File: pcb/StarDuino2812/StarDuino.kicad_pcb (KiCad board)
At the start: 2 copper layers, 126.3 x 120.3 mm, 68 parts, among them J1 Screw_Terminal_01x02, Q1 IRLML6401, U1 ATmega328P-AU, Y1 Crystal

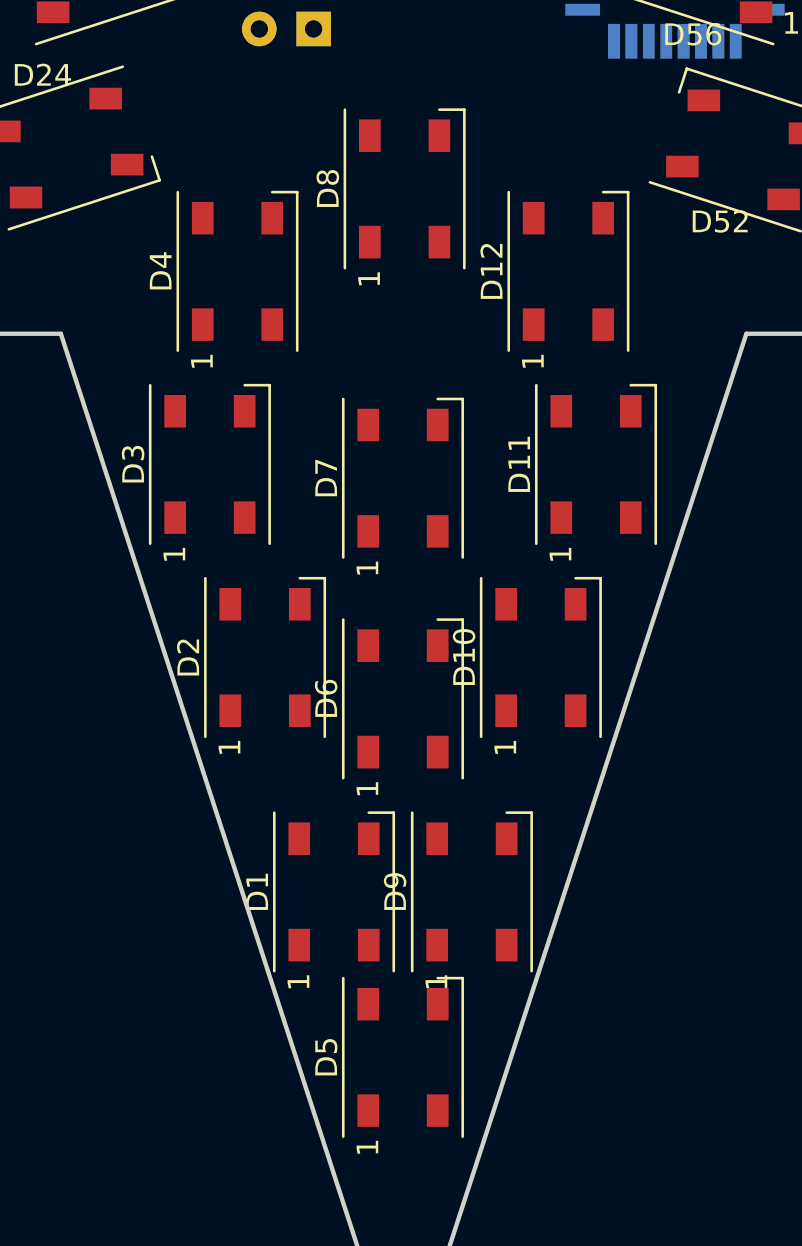
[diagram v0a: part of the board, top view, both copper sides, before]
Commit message: 2812 star in work
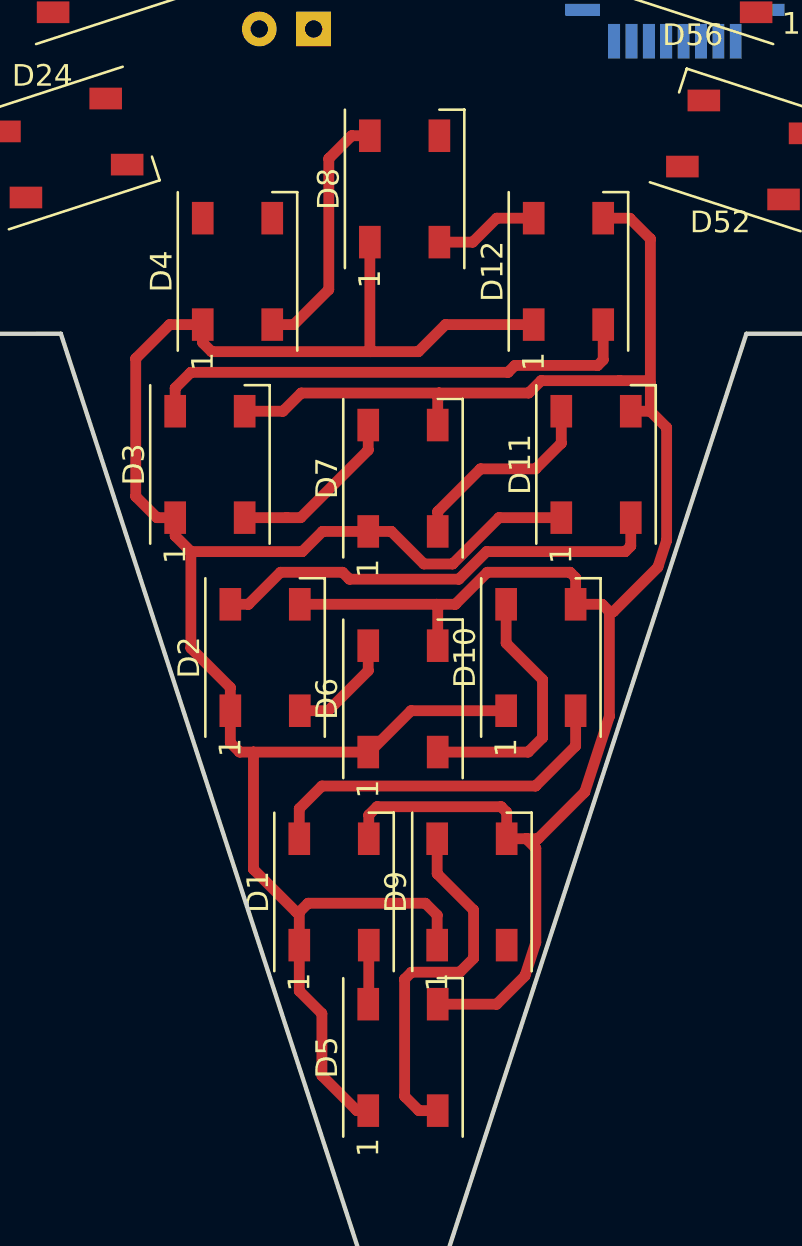
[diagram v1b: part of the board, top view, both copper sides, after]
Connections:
- D10 pad 2: Net-(D10-Pad2) -> Net-(D1-Pad4)
- D11 pad 4: Net-(D10-Pad2) -> Net-(D11-Pad4)
- D12 pad 4: Net-(D11-Pad2) -> Net-(D12-Pad4)
- D14 pad 4: Net-(D13-Pad2) -> Net-(D14-Pad4)
- D15 pad 4: Net-(D14-Pad2) -> Net-(D15-Pad4)
- D16 pad 4: Net-(D15-Pad2) -> Net-(D16-Pad4)
- D18 pad 4: Net-(D17-Pad2) -> Net-(D18-Pad4)
- D19 pad 4: Net-(D18-Pad2) -> Net-(D19-Pad4)
- D2 pad 4: Net-(D1-Pad2) -> Net-(D11-Pad2)
- D20 pad 4: Net-(D19-Pad2) -> Net-(D20-Pad4)
- D22 pad 4: Net-(D21-Pad2) -> Net-(D22-Pad4)
- D23 pad 4: Net-(D22-Pad2) -> Net-(D23-Pad4)
- D24 pad 4: Net-(D23-Pad2) -> Net-(D24-Pad4)
- D26 pad 4: Net-(D25-Pad2) -> Net-(D26-Pad4)
- D27 pad 4: Net-(D26-Pad2) -> Net-(D27-Pad4)
- D28 pad 4: Net-(D27-Pad2) -> Net-(D28-Pad4)
- D3 pad 4: Net-(D2-Pad2) -> Net-(D12-Pad2)
- D30 pad 4: Net-(D29-Pad2) -> Net-(D30-Pad4)
- D31 pad 4: Net-(D30-Pad2) -> Net-(D31-Pad4)
- D32 pad 4: Net-(D31-Pad2) -> Net-(D32-Pad4)
- D34 pad 4: Net-(D33-Pad2) -> Net-(D34-Pad4)
- D35 pad 4: Net-(D34-Pad2) -> Net-(D35-Pad4)
- D36 pad 4: Net-(D35-Pad2) -> Net-(D36-Pad4)
- D38 pad 4: Net-(D37-Pad2) -> Net-(D38-Pad4)
- D39 pad 4: Net-(D38-Pad2) -> Net-(D39-Pad4)
- D4 pad 4: Net-(D3-Pad2) -> Net-(D4-Pad4)
- D40 pad 4: Net-(D39-Pad2) -> Net-(D40-Pad4)
- D42 pad 4: Net-(D41-Pad2) -> Net-(D42-Pad4)
- D43 pad 4: Net-(D42-Pad2) -> Net-(D43-Pad4)
- D44 pad 4: Net-(D43-Pad2) -> Net-(D44-Pad4)
- D46 pad 4: Net-(D45-Pad2) -> Net-(D46-Pad4)
- D47 pad 4: Net-(D46-Pad2) -> Net-(D47-Pad4)
- D48 pad 4: Net-(D47-Pad2) -> Net-(D48-Pad4)
- D5 pad 4: Net-(D5-Pad4) -> Net-(D1-Pad2)
- D50 pad 4: Net-(D49-Pad2) -> Net-(D50-Pad4)
- D51 pad 4: Net-(D50-Pad2) -> Net-(D51-Pad4)
- D52 pad 4: Net-(D51-Pad2) -> Net-(D52-Pad4)
- D54 pad 4: Net-(D53-Pad2) -> Net-(D54-Pad4)
- D55 pad 4: Net-(D54-Pad2) -> Net-(D55-Pad4)
- D56 pad 4: Net-(D55-Pad2) -> Net-(D56-Pad4)
- D58 pad 4: Net-(D57-Pad2) -> Net-(D58-Pad4)
- D59 pad 4: Net-(D58-Pad2) -> Net-(D59-Pad4)
- D6 pad 2: Net-(D6-Pad2) -> Net-(D10-Pad4)
- D6 pad 4: Net-(D5-Pad2) -> Net-(D2-Pad2)
- D60 pad 4: Net-(D59-Pad2) -> Net-(D60-Pad4)
- D7 pad 2: Net-(D7-Pad2) -> Net-(D11-Pad4)
- D7 pad 4: Net-(D6-Pad2) -> Net-(D3-Pad2)
- D8 pad 2: Net-(D8-Pad2) -> Net-(D12-Pad4)
- D8 pad 4: Net-(D7-Pad2) -> Net-(D4-Pad2)
- D9 pad 2: Net-(D10-Pad4) -> Net-(D9-Pad2)
- D9 pad 4: Net-(D9-Pad4) -> Net-(D5-Pad2)
- U1 pad 7: Net-(U1-Pad7) -> Net-(C2-Pad1)
- U1 pad 8: Net-(U1-Pad8) -> Net-(C1-Pad1)
- Y1 pad 1: Net-(Y1-Pad1) -> Net-(C1-Pad1)
- Y1 pad 2: Net-(Y1-Pad2) -> Net-(C2-Pad1)
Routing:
- net VCC: track 0.00 -> 105.4 mm
- net GND: track 0.00 -> 94.2 mm
- net Net-(D12-Pad2): track 0.00 -> 22.9 mm
- net Net-(D11-Pad2): track 0.00 -> 21.1 mm
- net Net-(D5-Pad2): track 0.00 -> 17.0 mm
- net Net-(D1-Pad4): track 0.00 -> 16.9 mm
- net Net-(D10-Pad4): track 0.00 -> 11.9 mm
- net Net-(D4-Pad2): track 0.00 -> 11.6 mm
- net Net-(D11-Pad4): track 0.00 -> 9.38 mm
- net Net-(D3-Pad2): track 0.00 -> 8.13 mm
- net Net-(D2-Pad2): track 0.00 -> 5.07 mm
- net Net-(D12-Pad4): track 0.00 -> 4.80 mm
- net Net-(D1-Pad2): track 0.00 -> 2.73 mm
